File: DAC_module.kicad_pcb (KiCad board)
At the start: 2 copper layers, 22.1 x 19.9 mm, 21 parts, among them J2 Conn_01x05_Pin, J3 Conn_01x05_Pin, J5 Conn_02x04_Counter_Clockwise, U2 DAC80504

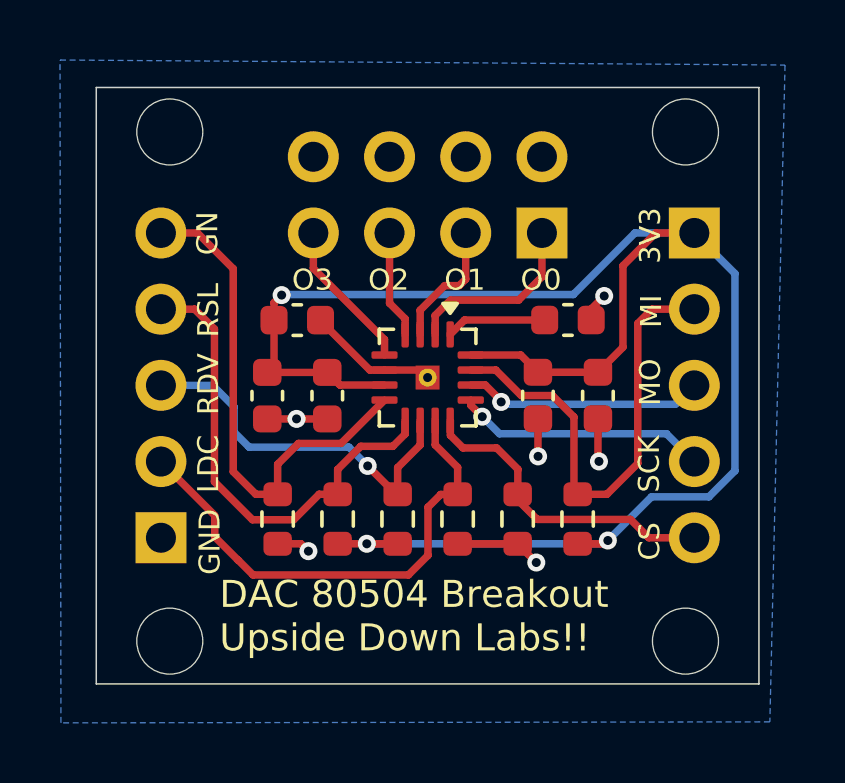
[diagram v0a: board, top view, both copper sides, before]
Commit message: Adding files of PCB v0.2
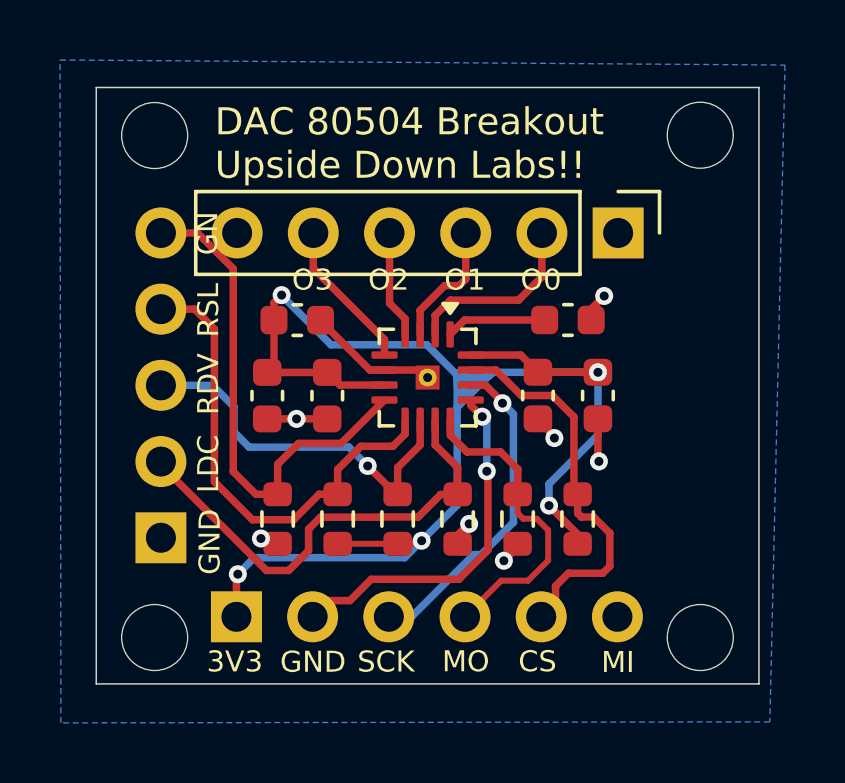
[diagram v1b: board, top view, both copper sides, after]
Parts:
- removed J5: Conn_02x04_Counter_Clockwise, Connector_PinHeader_2.54mm:PinHeader_2x04_P2.54mm_Vertical
- added J1: Conn_01x06_Pin, Connector_PinHeader_2.54mm:PinHeader_1x06_P2.54mm_Vertical, F.Cu at (75.2, 32.0)
- J2: value Conn_01x05_Pin -> Conn_01x06_Pin; footprint Connector_PinHeader_2.54mm:PinHeader_1x05_P2.54mm_Vertical -> Connector_PinHeader_2.54mm:PinHeader_1x06_P2.54mm_Vertical
- moved J2 19.9 mm to (62.5, 44.8), turned to -90 degrees
- moved H4 0.52 mm to (59.8, 45.5)
- moved H3 0.52 mm to (59.8, 28.8)
- moved H1 0.51 mm to (78.0, 45.5)
- moved H2 0.51 mm to (78.0, 28.8)
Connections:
- J2 pad 2: /MISO -> /SCLK
- J2 pad 4: /SCLK -> /CS
- J2 pad 5: /CS -> /MISO
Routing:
- net +3V3: track 57.2 -> 47.9 mm, vias 3 -> 5
- net /SCLK: track 8.40 -> 12.0 mm, vias 1 -> 2
- net /MOSI: track 8.00 -> 11.0 mm
- net /MISO: track 15.7 -> 13.2 mm
- net GND: track 13.7 -> 11.6 mm, vias 6 -> 7
- net /LDAC: track 16.7 -> 15.7 mm
